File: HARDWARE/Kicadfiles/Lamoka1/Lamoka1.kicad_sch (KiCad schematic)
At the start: 8 parts, among them J1 2606-1108/010-000, J2 2606-1352, J3 USB_C_Receptacle_USB2.0_14P, J4 470531000, J5 2604-1103

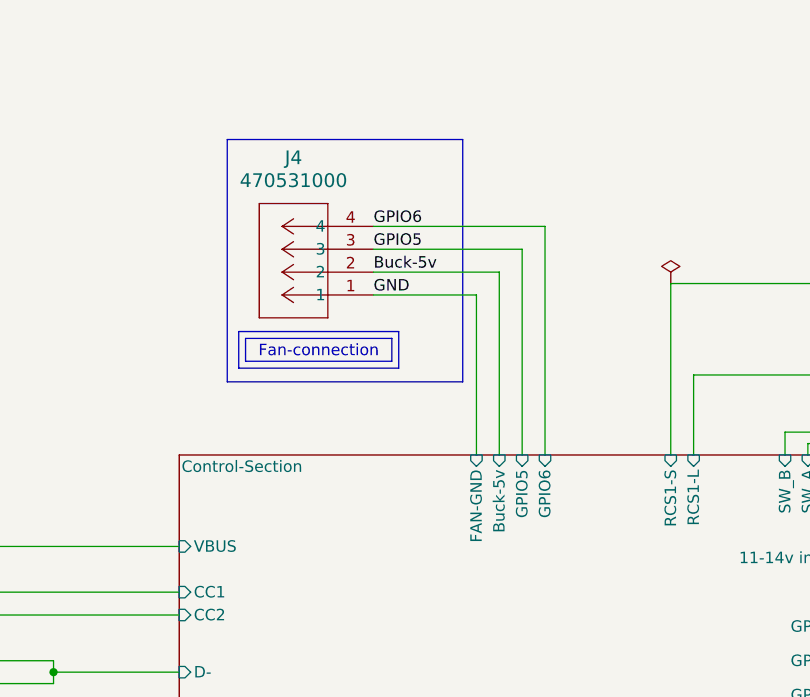
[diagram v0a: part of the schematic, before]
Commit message: MOSFET ROUTING, AND SUCH
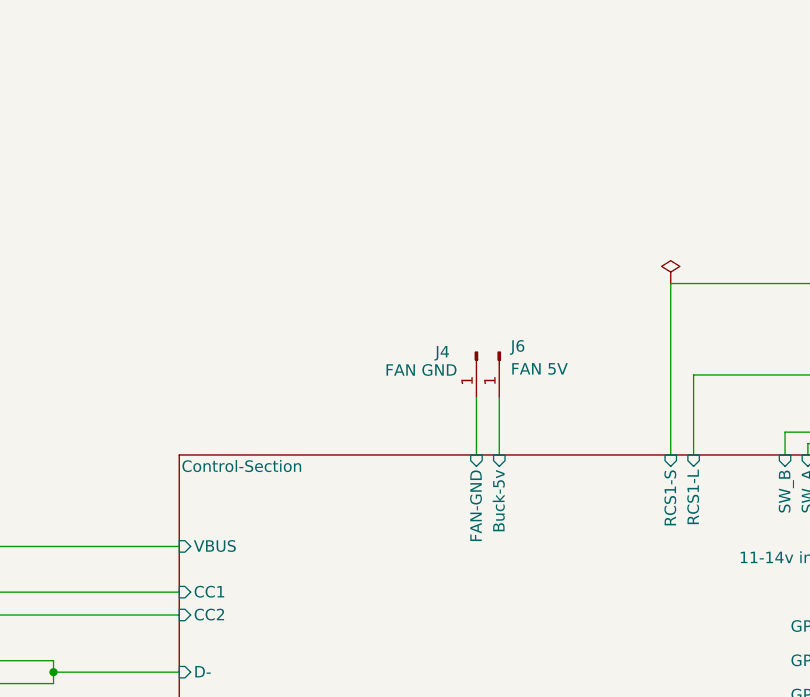
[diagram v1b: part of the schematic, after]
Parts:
- removed J4: 470531000, Connector:FanPinHeader_1x04_P2.54mm_Vertical, symbol 470531000:470531000
- added J4: FAN GND, Connector_Wire:SolderWirePad_1x01_SMD_3x6mm, symbol Connector:Conn_01x01_Pin
- added J6: FAN 5V, Connector_Wire:SolderWirePad_1x01_SMD_3x6mm, symbol Connector:Conn_01x01_Pin
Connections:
- new net Control-Section/Buck-5v: J6.1 (Pin_1)
- new net Control-Section/FAN-GND: J4.1 (Pin_1)
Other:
- sheet Control-Section ports: added none; removed GPIO5, GPIO6
- note removed: "Fan-connection"
